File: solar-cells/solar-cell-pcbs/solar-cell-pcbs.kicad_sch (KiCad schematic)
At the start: 7 parts, among them J1 4P2C

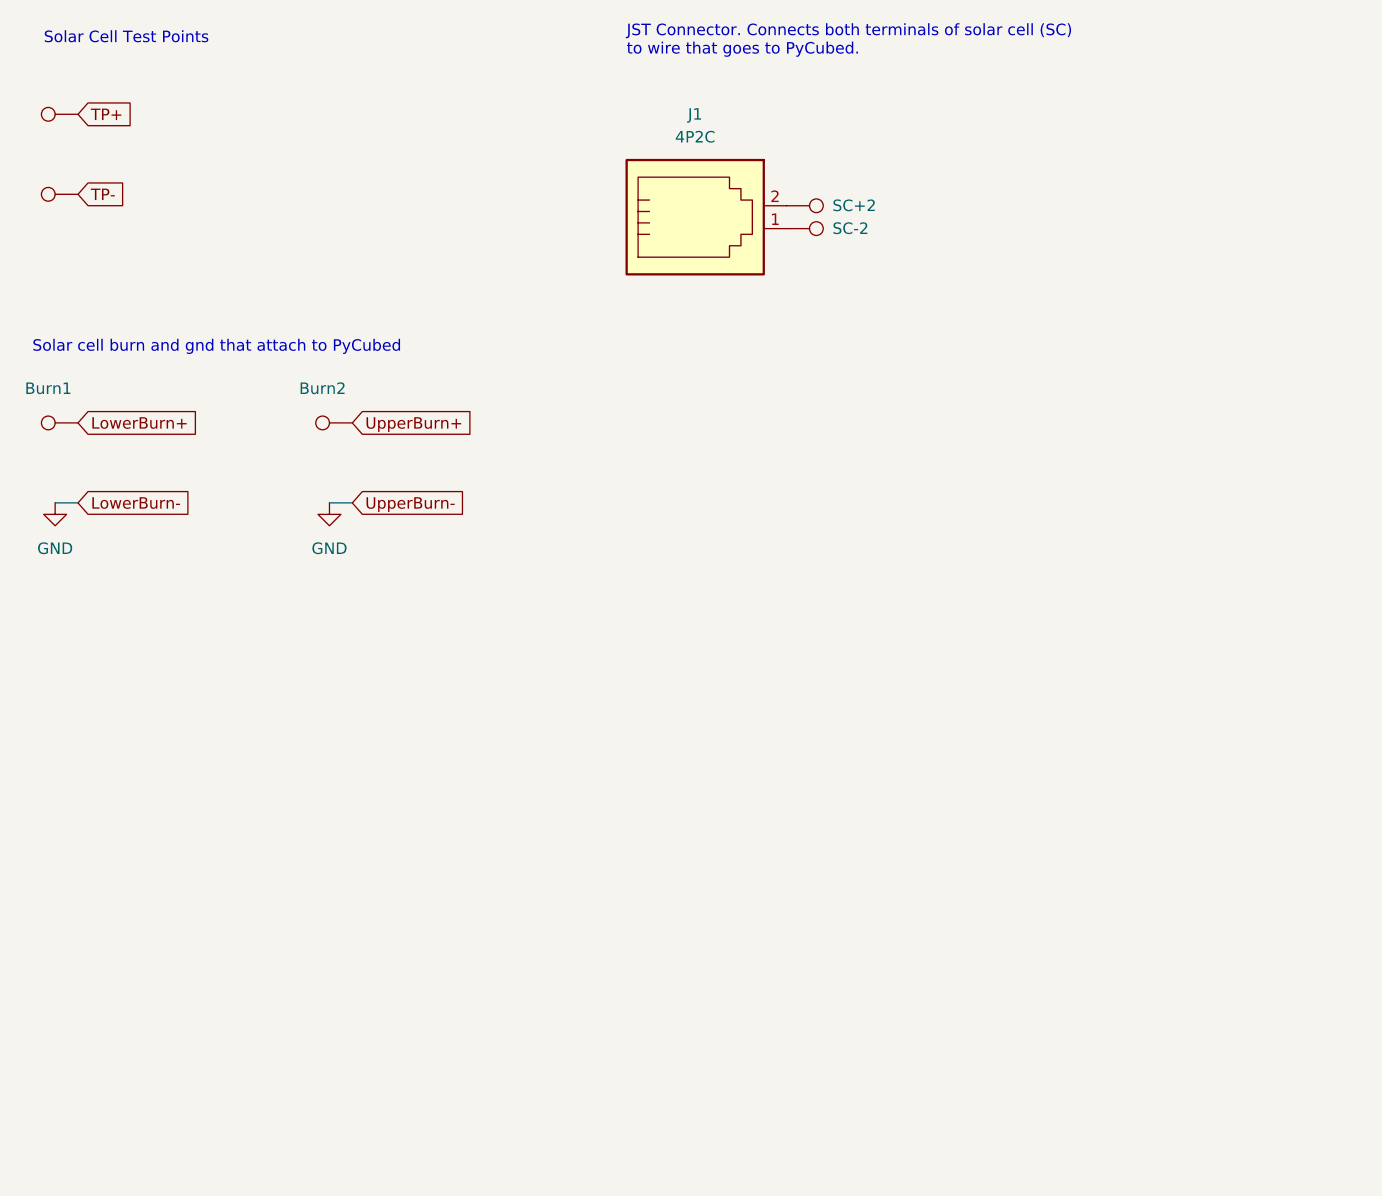
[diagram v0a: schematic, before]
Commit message: modifications to solar cell pcb
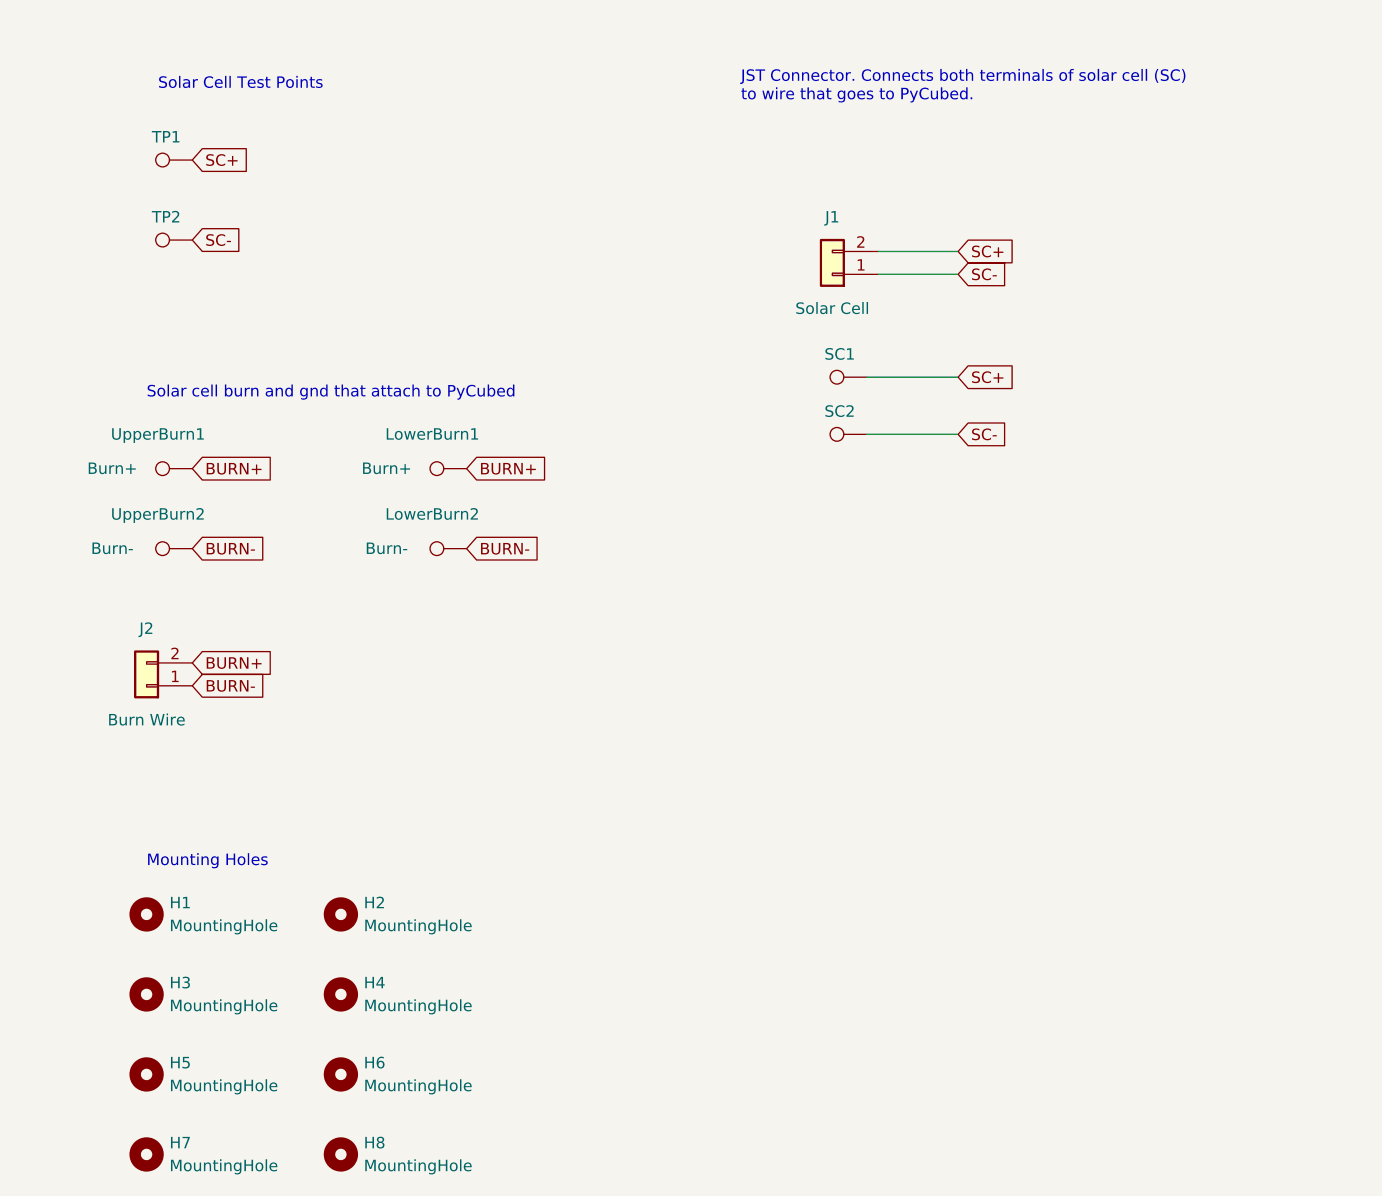
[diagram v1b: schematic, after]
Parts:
- removed J1: 4P2C, symbol Connector:4P2C
- added H1, H2, H3, H4, H5, H6, H7, H8: MountingHole, MountingHole:MountingHole_3.2mm_M3_DIN965_Pad, symbol Mechanical:MountingHole
- added J1: Solar Cell, Molex_PicoLock_2p_2mm_2053380002:2053380002, symbol Connector_Generic:Conn_01x02
- added J2: Burn Wire, Molex_PicoLock_2p_2mm_2053380002:2053380002, symbol Connector_Generic:Conn_01x02
- added LowerBurn2, UpperBurn2: Burn-, TestPoint:TestPoint_Pad_2.0x2.0mm, symbol Connector:TestPoint
- LowerBurn1: renamed from Burn2; value UpperBurn+ -> Burn+; footprint (none) -> TestPoint:TestPoint_Pad_2.0x2.0mm
- SC1: renamed from SC+2; footprint (none) -> TestPoint:TestPoint_Pad_D3.0mm
- SC2: renamed from SC-2; footprint (none) -> TestPoint:TestPoint_Pad_D3.0mm
- TP1: renamed from SC+1; footprint (none) -> TestPoint:TestPoint_Loop_D1.80mm_Drill1.0mm_Beaded; DNP (none) -> DNP
- TP2: renamed from SC-1; footprint (none) -> TestPoint:TestPoint_Loop_D1.80mm_Drill1.0mm_Beaded; DNP (none) -> DNP
- UpperBurn1: renamed from Burn1; value LowerBurn+ -> Burn+; footprint (none) -> TestPoint:TestPoint_Pad_2.0x2.0mm
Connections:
- net TP+ is gone; now on net SC+: TP1.1
- net TP- is gone; now on net SC-: TP2.1
- net UpperBurn+ is gone; now on net BURN+: LowerBurn1.1
- net SC-: now reaches SC2.1
- net SC-: now also J1.1 (Pin_1)
- net SC+: now reaches SC1.1
- net SC+: now also J1.2 (Pin_2)
- net LowerBurn+ renamed BURN+
- net BURN+: now also J2.2 (Pin_2)
- new net BURN-: J2.1 (Pin_1), LowerBurn2.1, UpperBurn2.1
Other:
- note added: "Mounting Holes"
- moved on the sheet: LowerBurn1, SC1, SC2, UpperBurn1
